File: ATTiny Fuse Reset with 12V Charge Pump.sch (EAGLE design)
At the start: 35 parts, among them U2 ARDUINOR3-BPLACE

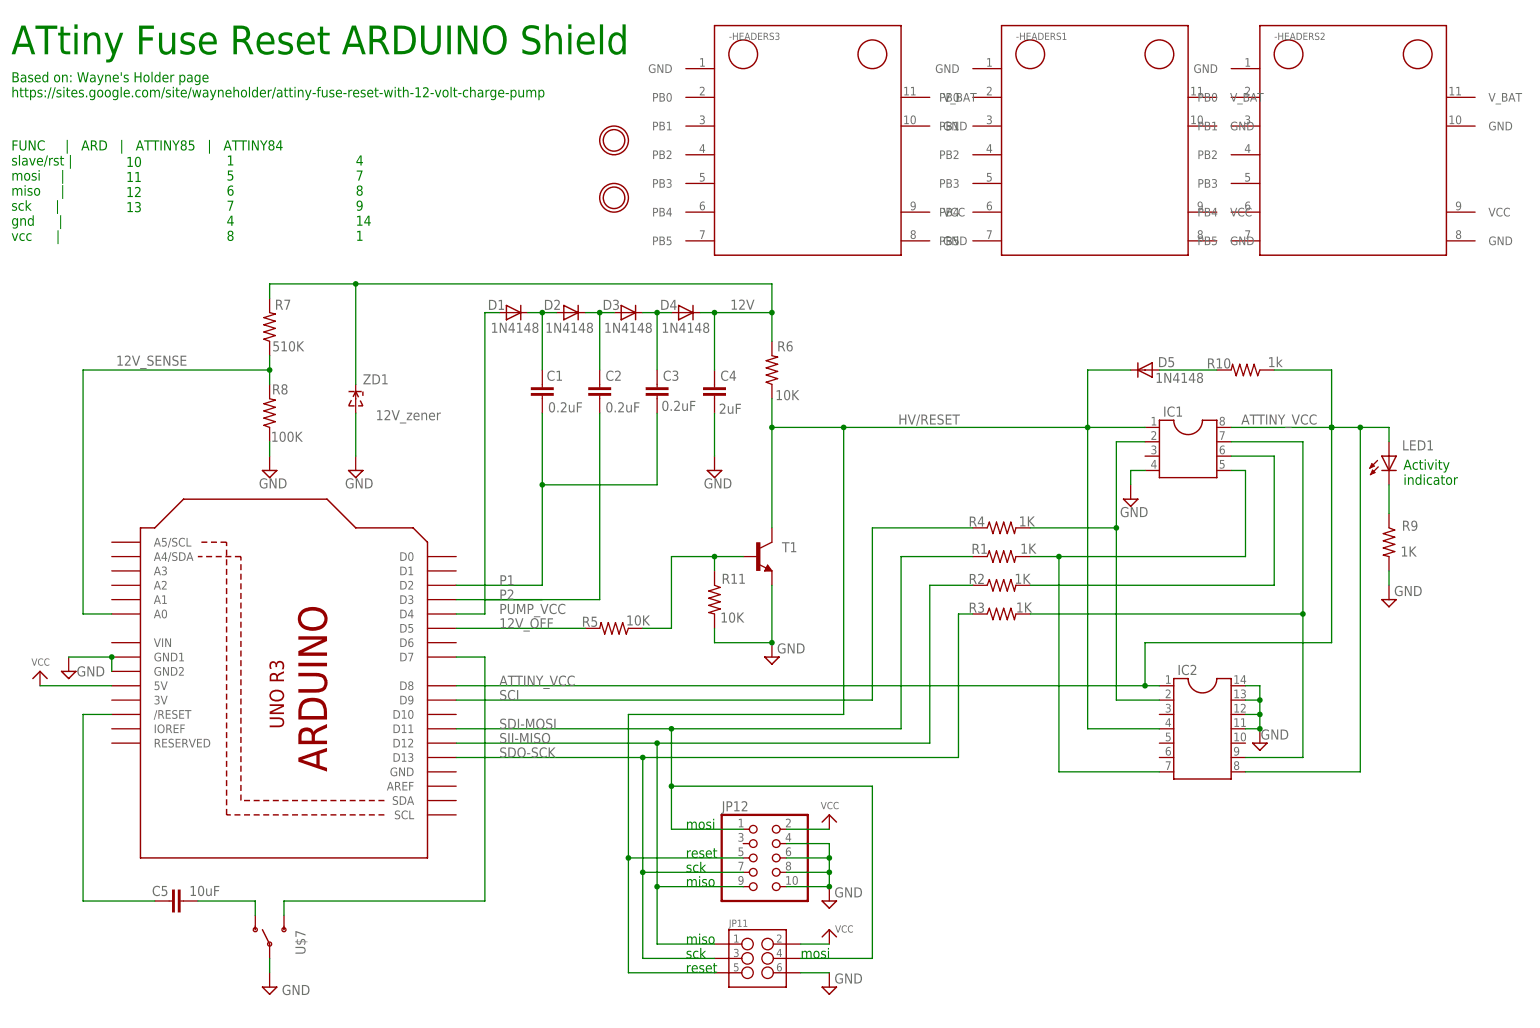
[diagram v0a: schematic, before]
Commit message: Changes in the schematic
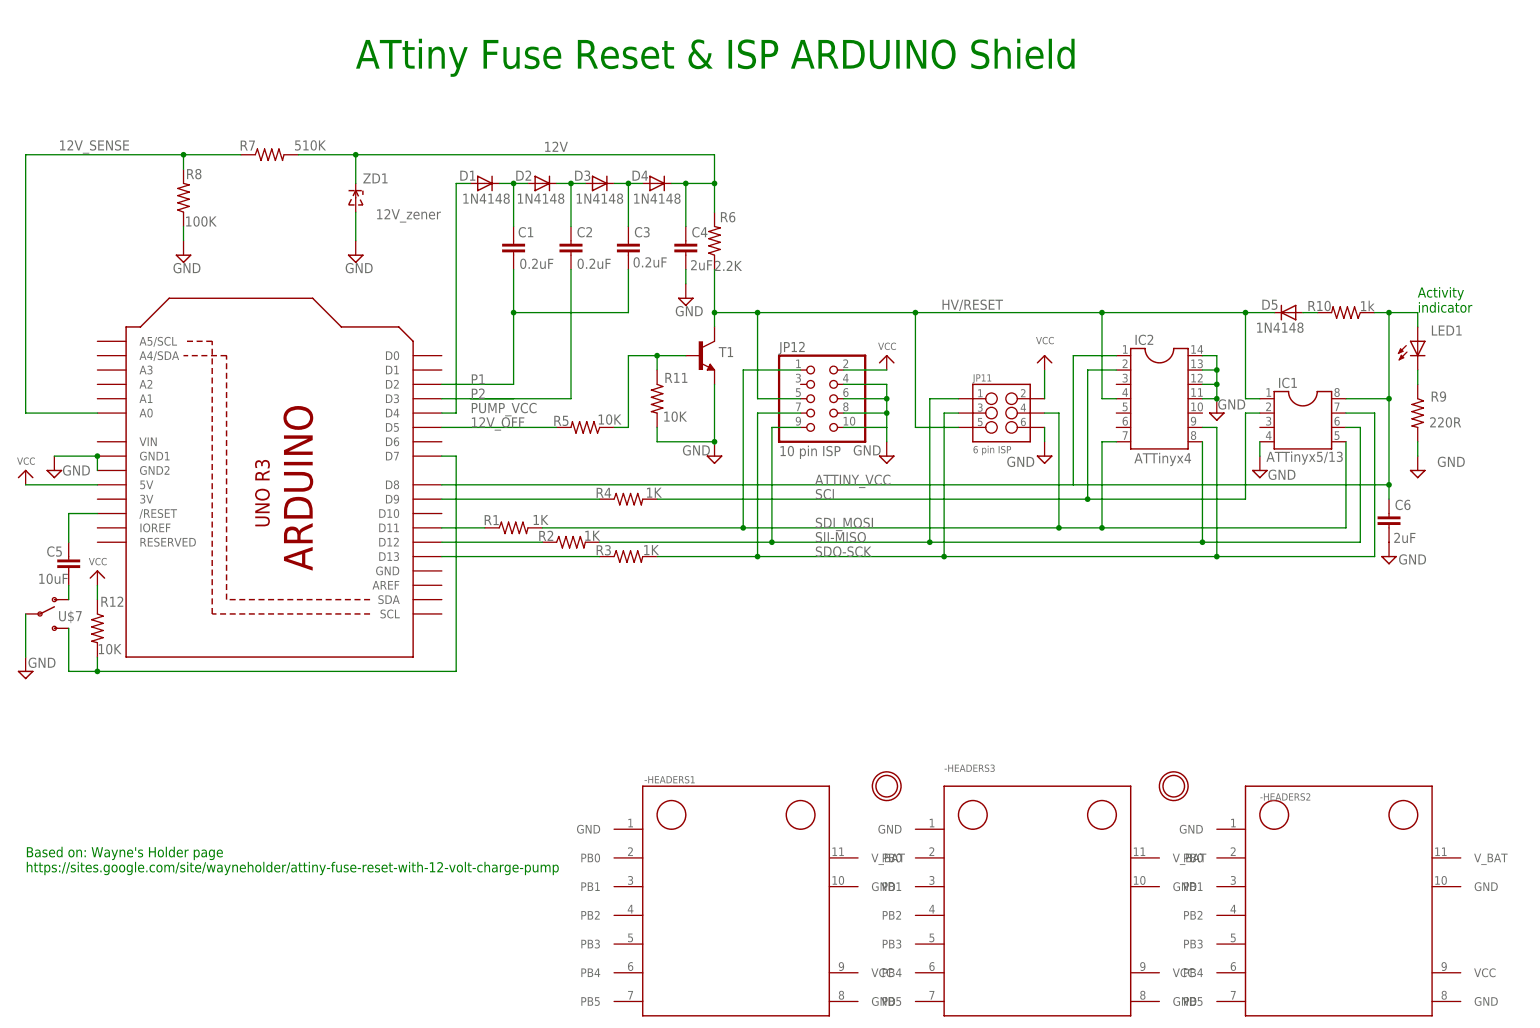
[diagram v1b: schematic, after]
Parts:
- added C6: 2uF, ATtami:CAP0805
- added R12: 10K, ATtami:RESISTOR0805-RES
- -HEADERS1: value (none) -> ATTami
- IC1: value (none) -> ATTinyx5/13
- IC2: value (none) -> ATTinyx4
- JP11: value (none) -> 6 pin ISP
- JP12: value (none) -> 10 pin ISP
- R6: value 10K -> 2.2K
- R9: value 1K -> 220R
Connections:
- removed net N$13: IC1.6, R2.2
- removed net N$14: IC1.2, IC2.2, R4.2
- removed net SDI-MOSI: JP11.4, JP12.1, R1.1, U2.D11
- new net N$21: R1.1, U2.D11
- new net N$7: R3.1, U2.D13
- new net SDI_MOSI: IC1.5, IC2.7, JP11.4, JP12.1, R1.2
- net ATTINY_VCC: now also C6.1; no longer IC2.8
- net GND: now also C6.2
- net N$2: now also R4.1, U2.D9; no longer IC1.5, IC2.7, R1.2
- net N$8: now also R2.1, U2.D12; no longer IC1.7, IC2.9, R3.2
- net N$9: now also R12.2
- net SCI: now also IC1.2, IC2.2, R4.2; no longer R4.1, U2.D9
- net SDO-SCK: now also IC1.7, IC2.9, R3.2; no longer R3.1, U2.D13
- net SII-MISO: now also IC1.6, IC2.8, R2.2; no longer R2.1, U2.D12
- net VCC: now also R12.1
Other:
- note added: "ATtiny Fuse Reset & ISP ARDUINO Shield"
- note removed: "1 5 6 7 4 8"
- note removed: "10 11 12 13"
- note removed: "4 7 8 9 14 1"
- note removed: "ATtiny Fuse Reset ARDUINO Shield"
- note removed: "FUNC | ARD | ATTINY85 | ATTINY84 slave/rst | mosi | miso | sck | gnd | vcc |"
- note removed: "miso"
- note removed: "mosi"
- note removed: "reset"
- note removed: "sck"
- moved on the sheet: -HEADERS1, -HEADERS2, -HEADERS3, C1, C2, C3, C4, C5, D1, D2, D3, D4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
